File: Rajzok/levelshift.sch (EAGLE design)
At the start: 17 parts, among them Q1 TP0602N2, Q2 TP0602N2, Q3 SUP75N06-08, Q4 SUP75N06-08

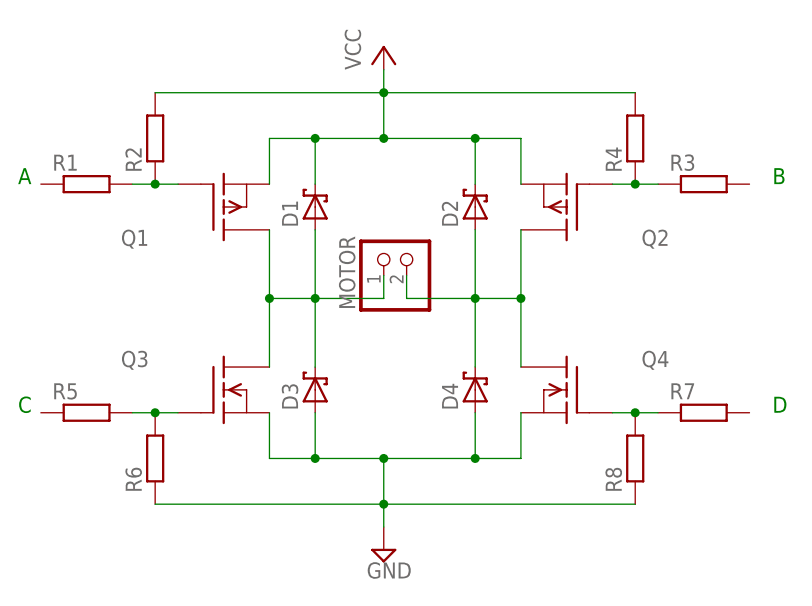
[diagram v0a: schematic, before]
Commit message: Rajzok 2017
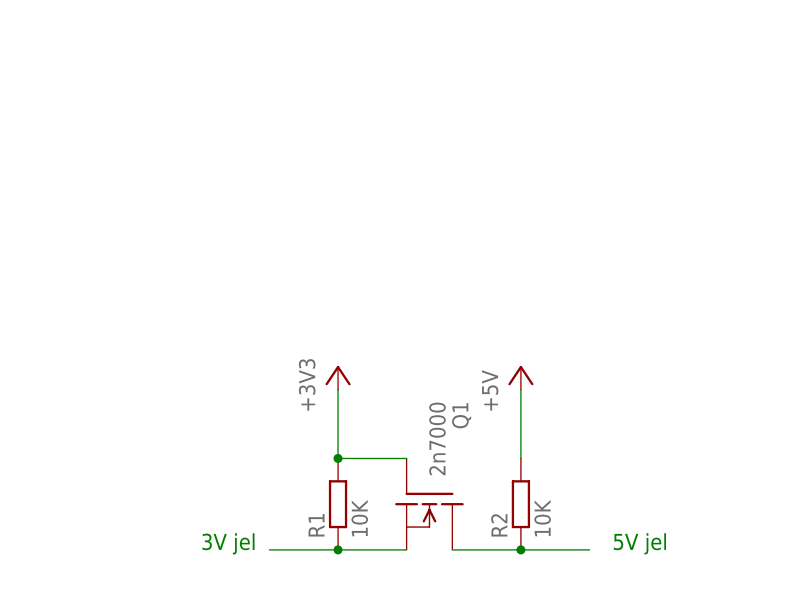
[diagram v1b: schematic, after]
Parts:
- removed D1, D2, D3, D4: 1N6267A, diode:1N6267A
- removed MOTOR: (no value), pinhead:PINHD-1X2
- removed Q2: TP0602N2, transistor-fet:TP0602N2
- removed Q3, Q4: SUP75N06-08, transistor-fet:SUP75N06-08
- removed R3, R4, R5, R6, R7, R8: (no value), rcl:R-EU_0204/7
- Q1: value TP0602N2 -> 2n7000; device transistor-fet:TP0602N2 -> transistor-fet:BSS97
- R1, R2: value (none) -> 10K; device rcl:R-EU_0204/7 -> rcl:R-EU_0309/12
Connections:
- removed net GND: D3.A, D4.A, Q3.S, Q4.S, R6.1, R8.1
- removed net N$3: Q2.G, R3.1, R4.1
- removed net N$4: Q3.G, R5.2, R6.2
- removed net N$5: Q4.G, R7.1, R8.2
- removed net N$9: D1.A, D3.C, MOTOR.1, Q1.D, Q3.D
- removed net VCC: D1.C, D2.C, Q1.S, Q2.S, R2.2, R4.2
- new net +3V3: Q1.G, R1.2
- new net +5V: R2.2
- net N$1: now also Q1.S, R1.1; no longer Q1.G, R1.2, R2.1
- net N$2: now also Q1.D, R2.1; no longer D2.A, D4.C, MOTOR.2, Q2.D, Q4.D
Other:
- note added: "3V jel"
- note added: "5V jel"
- note removed: "A"
- note removed: "B"
- note removed: "C"
- note removed: "D"
- moved on the sheet: Q1, R1, R2
